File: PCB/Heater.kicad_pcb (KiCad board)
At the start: 2 copper layers, 55 parts, among them IC1 ATTINY45-P, J1 GND, J2 RST, P1 220V 50Hz, P2 CONN_01X04, P3 DS18B20, U1 MOC3023M

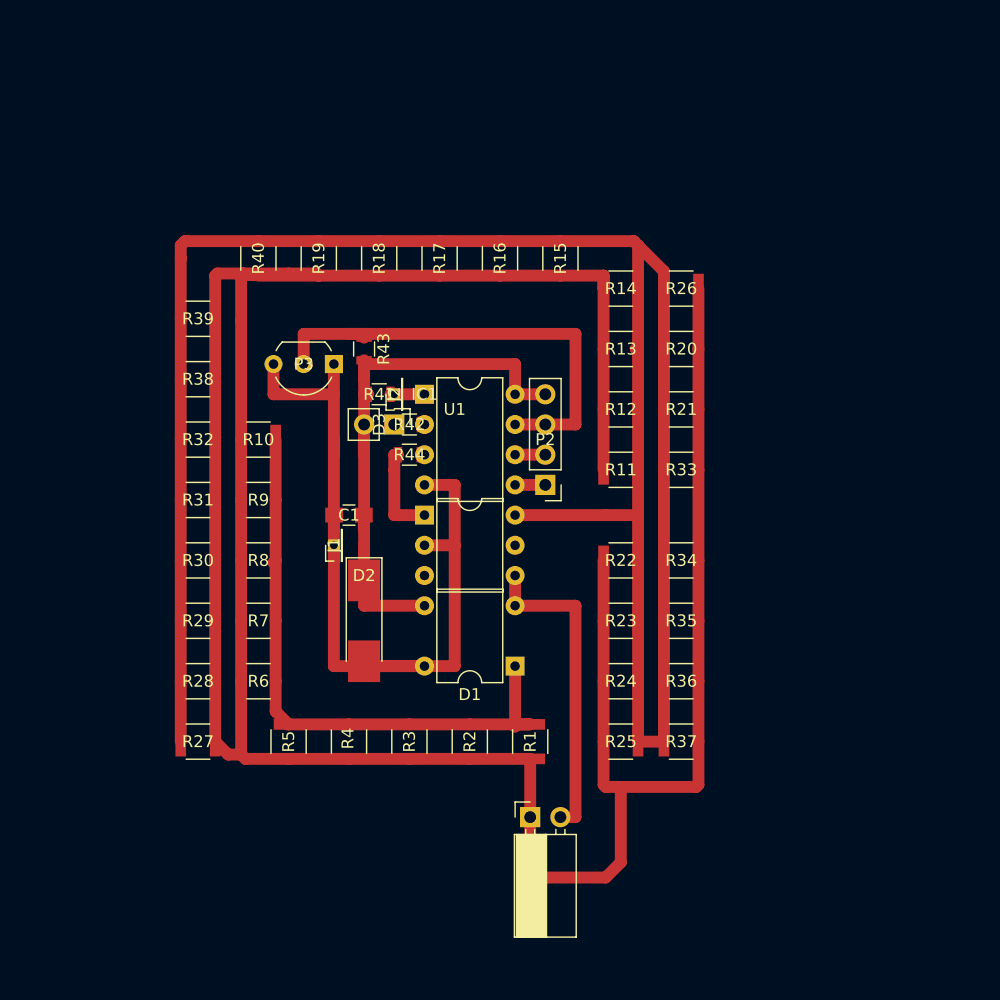
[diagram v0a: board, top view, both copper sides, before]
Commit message: Possible layout
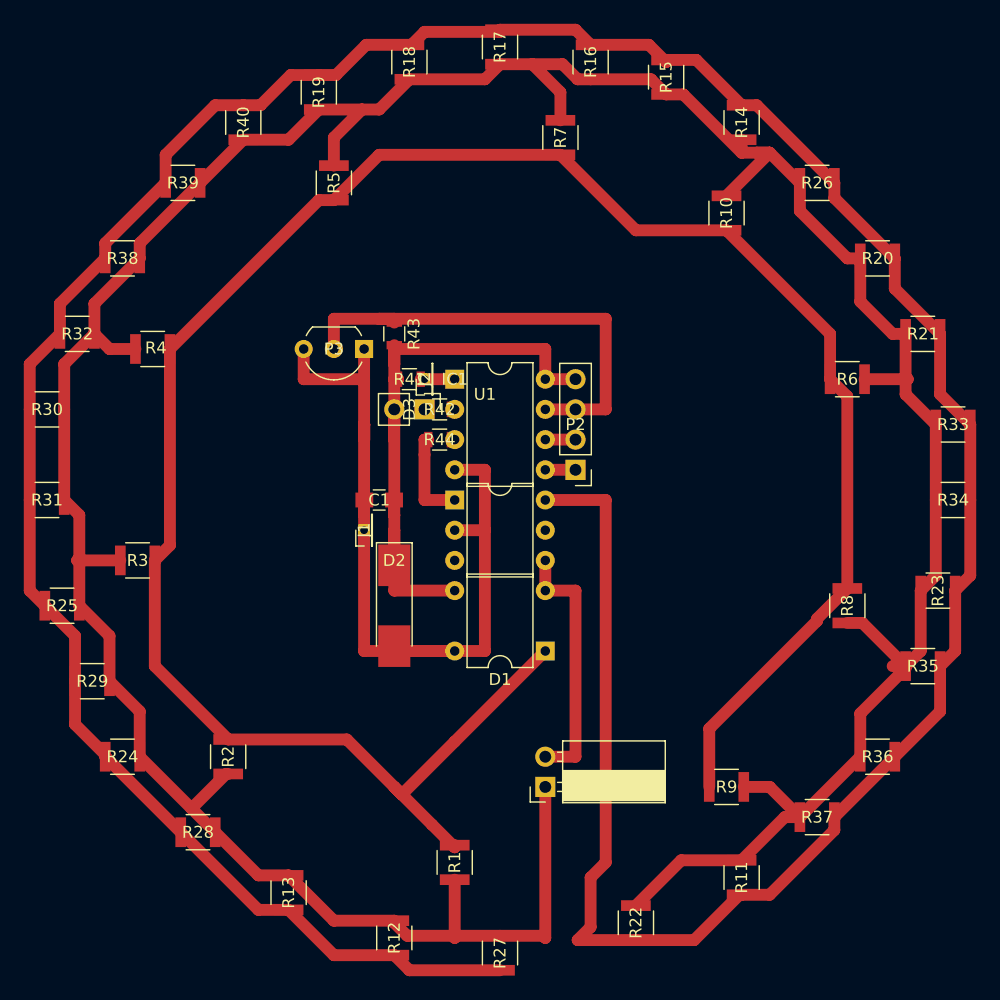
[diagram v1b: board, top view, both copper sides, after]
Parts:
- moved R6 55.7 mm to (105.4, 61.0), turned to 0 degrees
- moved R13 53.6 mm to (58.4, 104.1), turned to 90 degrees
- moved R8 49.7 mm to (105.4, 80.0), turned to 270 degrees
- moved R12 48.4 mm to (67.3, 108.0), turned to 90 degrees
- moved R25 48.4 mm to (39.4, 80.0), turned to 0 degrees
- moved R7 47.9 mm to (81.3, 40.6), turned to 90 degrees
- moved R5 47.1 mm to (62.2, 44.5), turned to 90 degrees
- moved R9 46.2 mm to (95.2, 95.2), turned to 0 degrees
- moved R10 43.7 mm to (95.2, 47.0), turned to 90 degrees
- moved R24 42.4 mm to (44.5, 92.7), turned to 0 degrees
- moved R4 36.9 mm to (47.0, 58.4), turned to 180 degrees
- moved R11 35.8 mm to (96.5, 102.9), turned to 90 degrees
- moved R27 31.0 mm to (76.2, 109.2), turned to 90 degrees
- moved R22 30.5 mm to (87.6, 106.7), turned to 90 degrees
- moved R3 27.5 mm to (45.7, 76.2), turned to 180 degrees
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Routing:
- net Net-(D1-Pad1): track 51.7 -> 188.9 mm
- net Net-(R11-Pad1): track 177.8 -> 297.3 mm
- net Net-(P1-Pad1): track 255.3 -> 301.5 mm
- net Net-(D1-Pad2): track 26.7 -> 21.6 mm
